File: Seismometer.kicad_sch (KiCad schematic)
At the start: 66 parts, among them U1 DLVR-F50D, U2 MC3479, U3 ADS131M04-Q1, U5 Teensy4.1, X1 SIT8924BA-22-33E-8.192000G

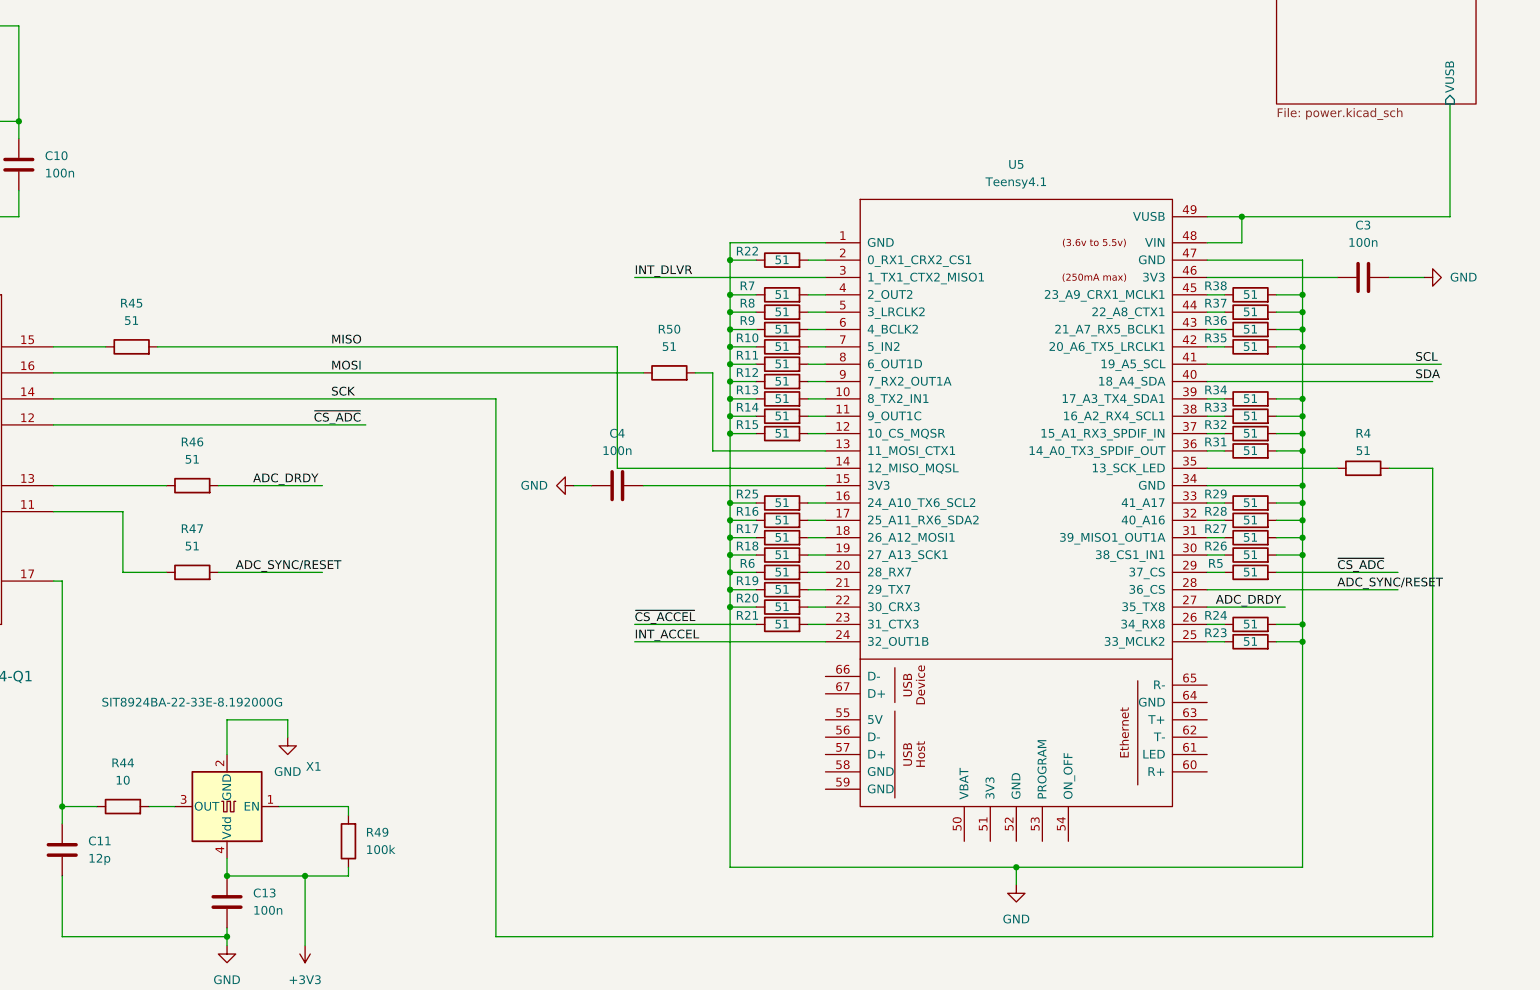
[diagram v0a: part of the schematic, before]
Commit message: wip Layout
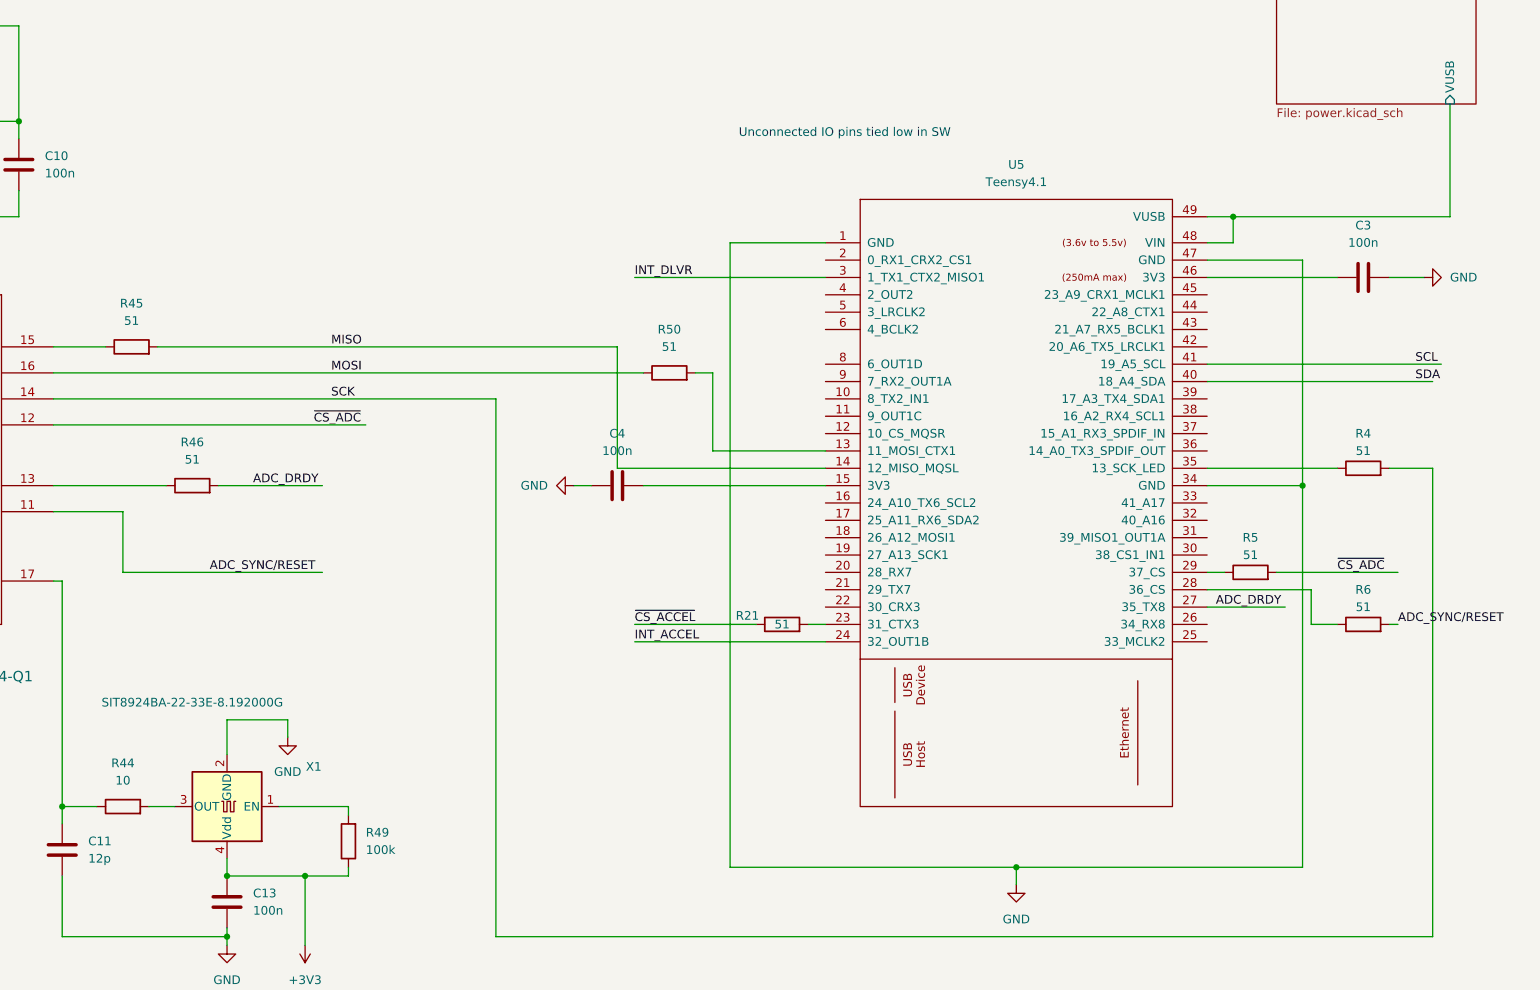
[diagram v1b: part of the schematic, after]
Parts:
- removed R10, R11, R12, R13, R14, R15, R16, R17, R18, R19, R20, R22, R23, R24, R25, R26, R27, R28, R29, R31, R32, R33, R34, R35, R36, R37, R38, R47, R7, R8, R9: 51, Resistor_SMD:R_0603_1608Metric, symbol Device:R
- C5, C9: footprint Capacitor_SMD:C_0805_2012Metric -> Capacitor_SMD:C_1206_3216Metric
- U2: Purchase-URL (none) -> https://www.snapeda.com/api/url_track_click_mouser/?unipart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; SnapEDA_Link (none) -> https://www.snapeda.com/parts/MC3479/Memsic/view-part/?ref=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
- U5: symbol seismometer:Teensy4.1 -> seismometer:Teensy4.1_minimal; now in the parts list
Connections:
- net ADC_SYNC/RESET: now also R6.2, U3.11 (SYNC/RESET); no longer U5.28 (36_CS)
- net GND: now also U5.52 (GND); no longer R6.1
- net at U5.20 (28_RX7): no longer R6.2
- new net: R6.1, U5.28 (36_CS)
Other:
- note added: "Unconnected IO pins tied low in SW"
